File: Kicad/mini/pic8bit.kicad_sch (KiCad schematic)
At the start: 11 parts, among them K101 PE-450-4X6X-BLACK

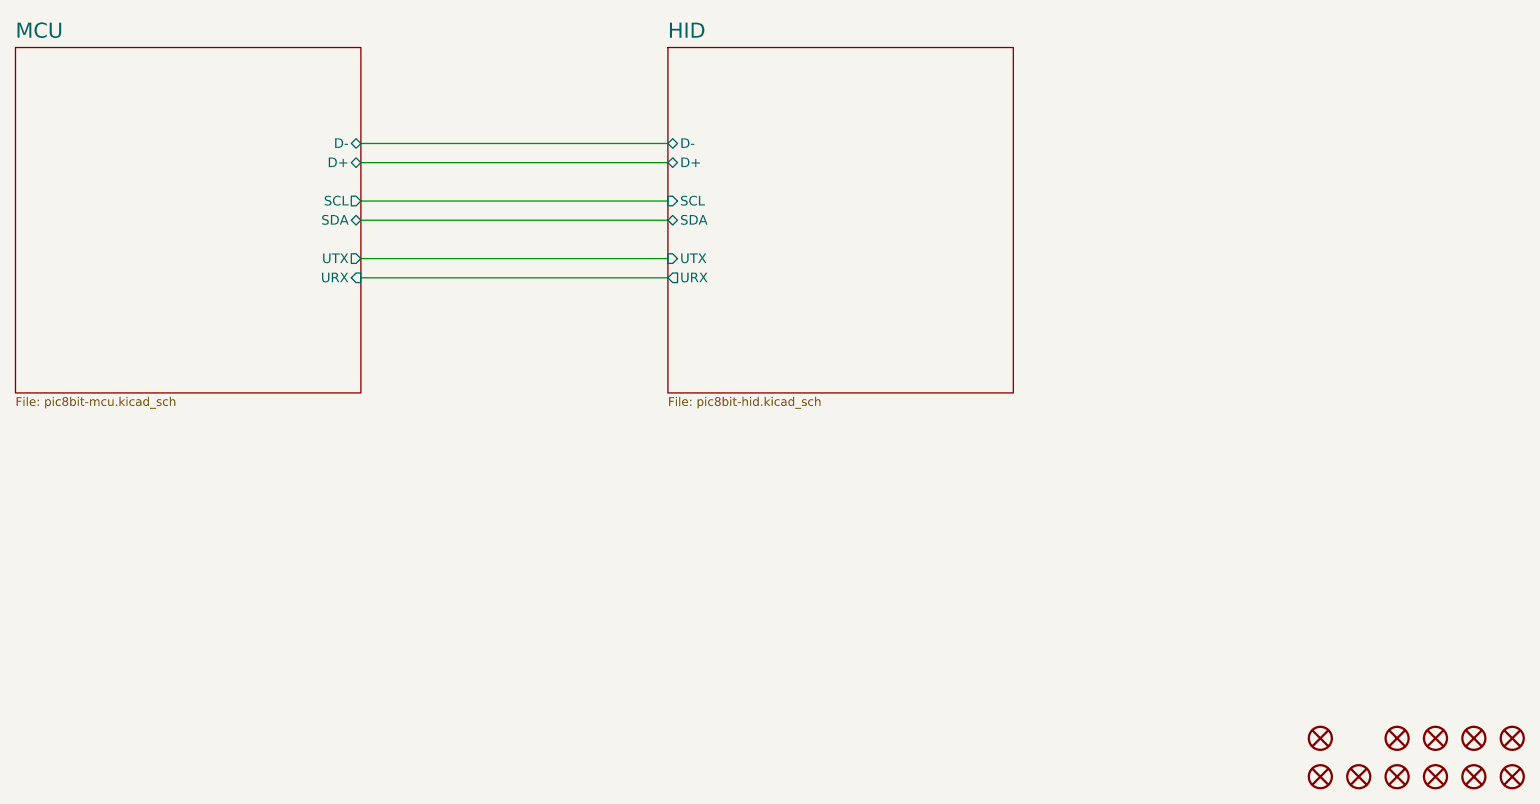
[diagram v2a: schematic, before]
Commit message: Update
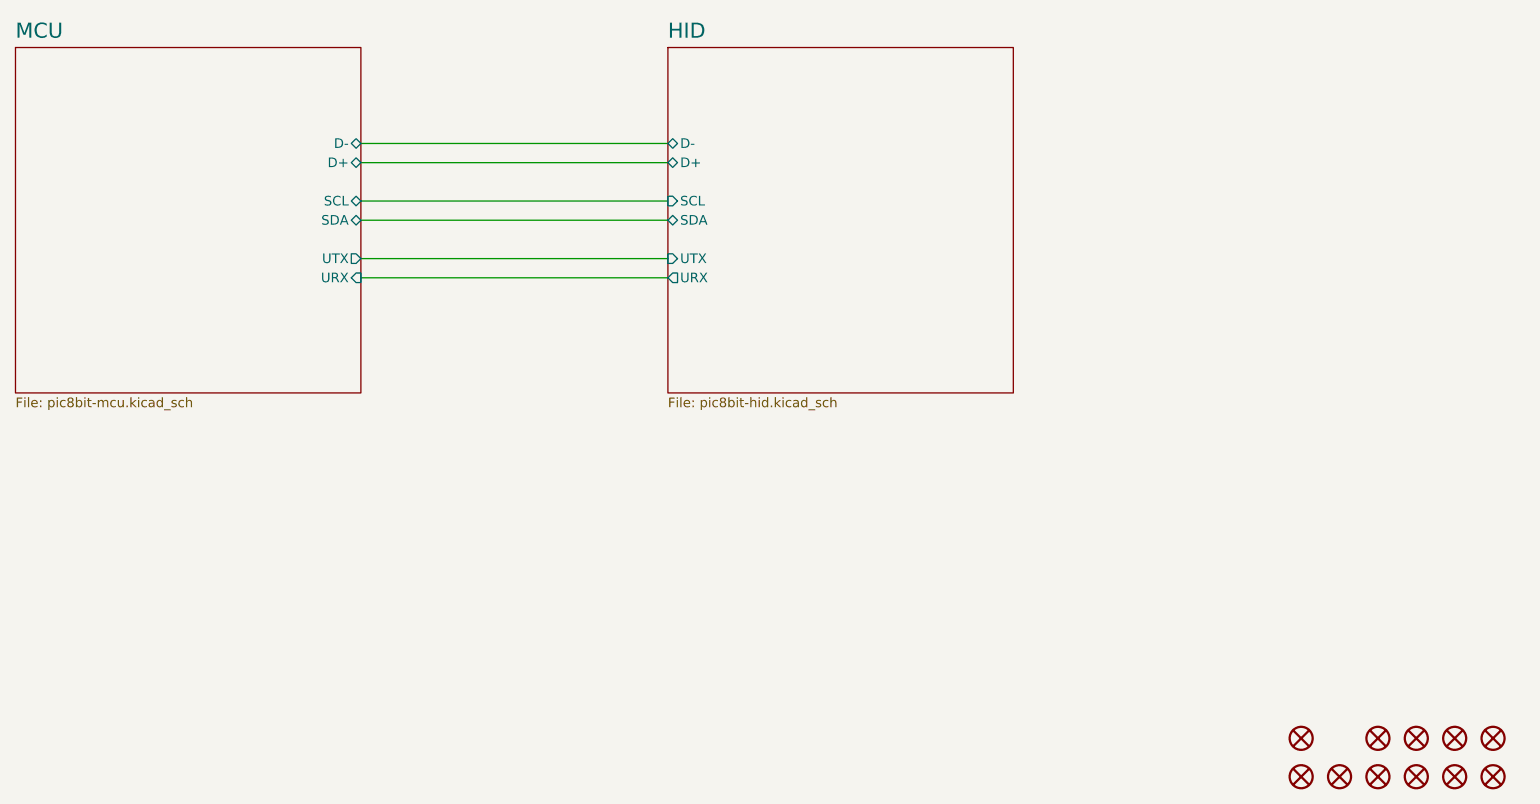
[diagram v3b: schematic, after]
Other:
- title: Diagram -> Connections
